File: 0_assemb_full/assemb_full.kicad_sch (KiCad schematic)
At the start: 4 parts, among them J1 Conn_01x02, J2 Conn_01x02, J3 Conn_01x02, U1 LM1117-3.3

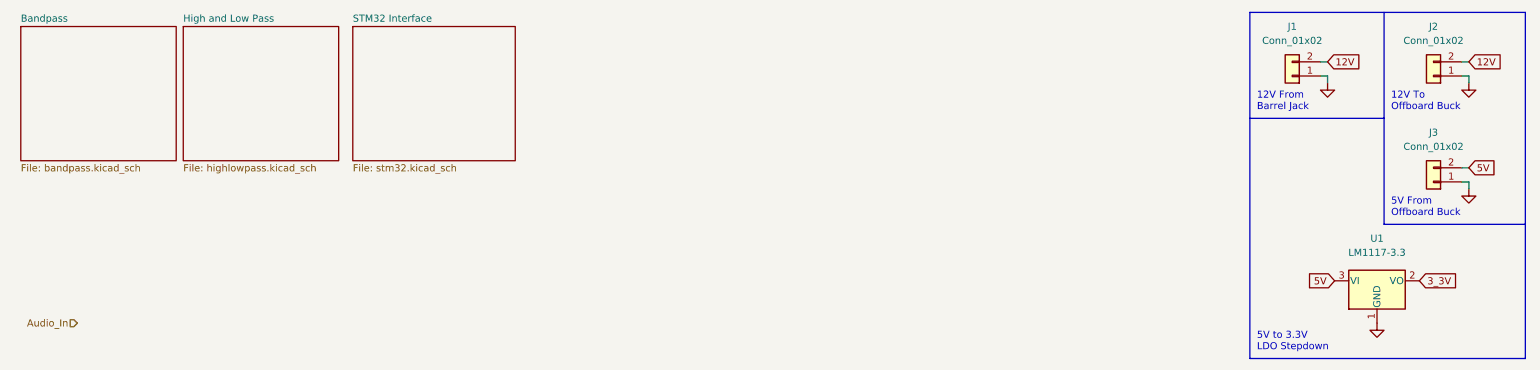
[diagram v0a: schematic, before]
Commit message: Additional changes
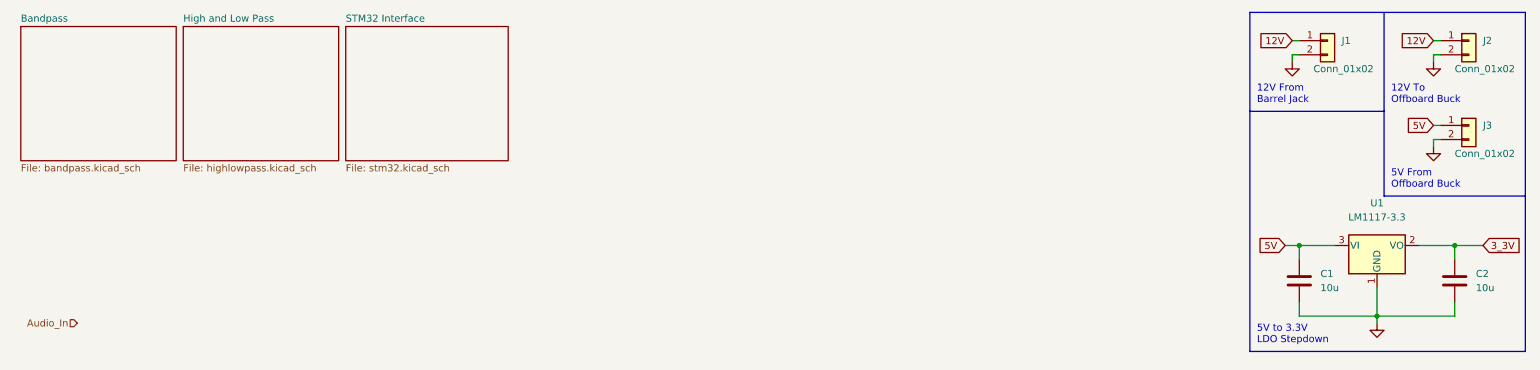
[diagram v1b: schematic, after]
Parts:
- added C1, C2: 10u, symbol Device:C
- J1: footprint (none) -> Connector_BarrelJack:BarrelJack_CUI_PJ-102AH_Horizontal
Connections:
- net 12V: now also J1.1 (Pin_1), J2.1 (Pin_1); no longer J1.2 (Pin_2), J2.2 (Pin_2)
- net 3_3V: now also C2.1
- net 5V: now also J3.1 (Pin_1), C1.1; no longer J3.2 (Pin_2)
- net GND: now also J1.2 (Pin_2), J2.2 (Pin_2), J3.2 (Pin_2), C1.2, C2.2; no longer J1.1 (Pin_1), J2.1 (Pin_1), J3.1 (Pin_1)
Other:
- moved on the sheet: J1, J2, J3, U1
